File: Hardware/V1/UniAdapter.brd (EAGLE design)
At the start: 30 x 21 mm, 24 parts, among them IC1 LD1117S33TR, IC2 SN65HVD232D, IC3 STM32F072CBT6, X1 CAN Bus, X2 CAN Bus

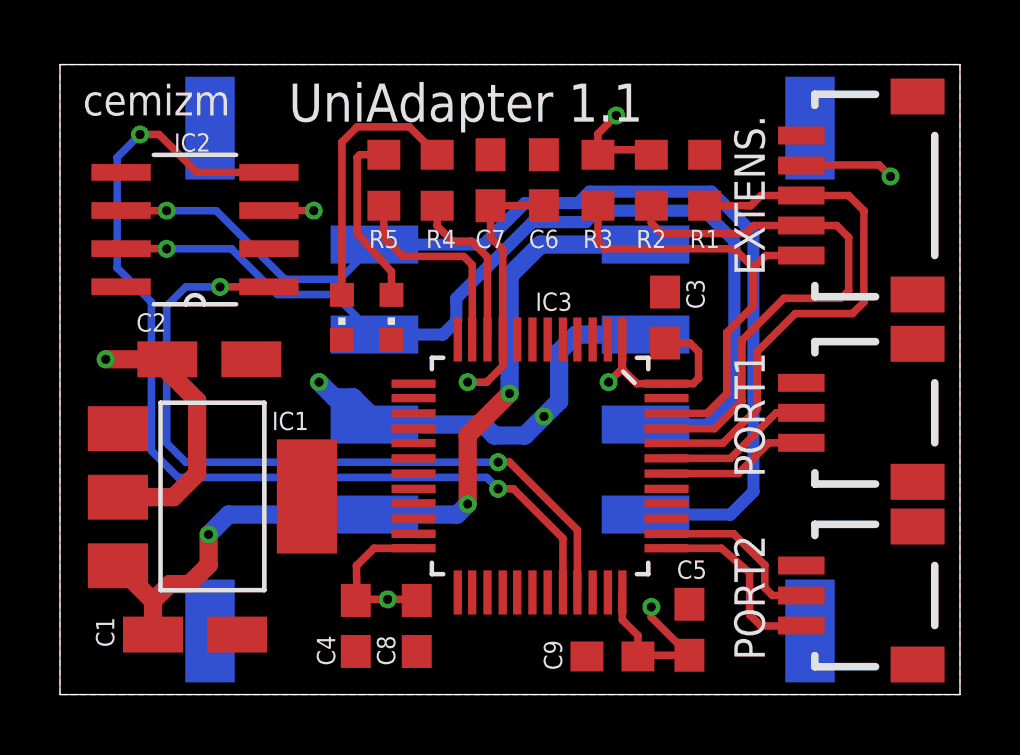
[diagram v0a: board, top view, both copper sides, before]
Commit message: AnySense 1.1
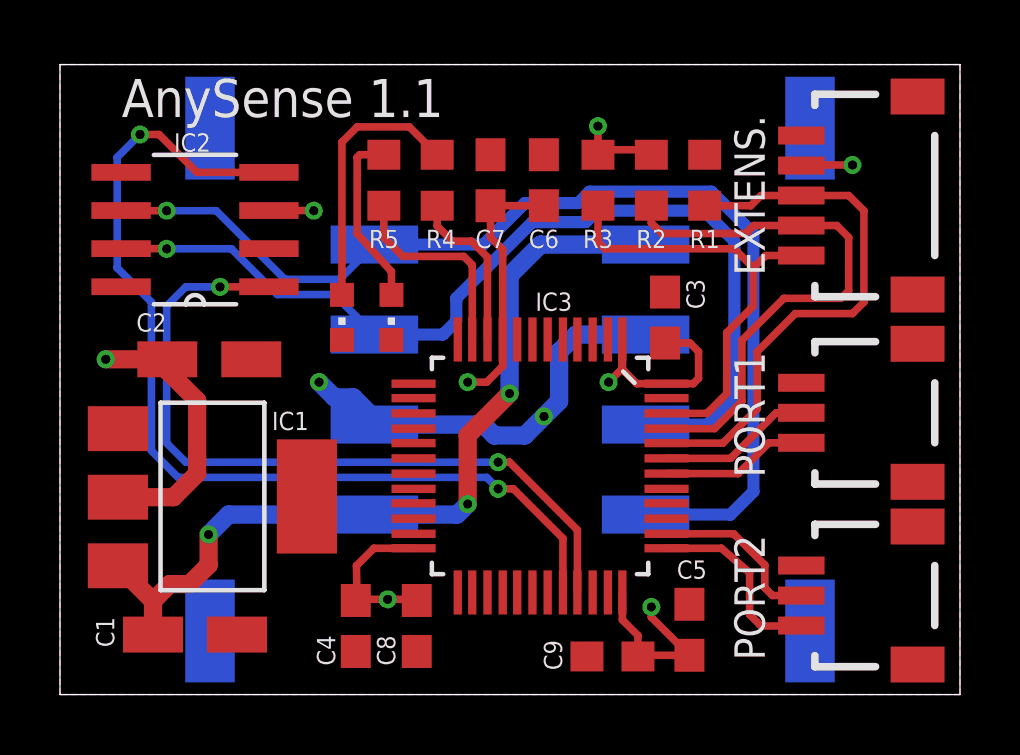
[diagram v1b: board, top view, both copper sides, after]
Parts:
- R4: value 55Ohm -> 68Ohm
- R5: value 55Ohm -> 56Ohm
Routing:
- net VCC: track 45.5 -> 43.4 mm
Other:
- board text added: "AnySense 1.1"
- board text removed: "UniAdapter 1.1"
- board text removed: "cemizm"
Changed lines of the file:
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@@
 <wire x1="22.7097375" y1="1.53345" x2="37.66655" y2="1.53345" width="0.254" layer="49"/>
 <wire x1="37.66655" y1="1.53345" x2="37.7" y2="1.5" width="0.254" layer="49" curve="-90"/>
-<text x="7.62" y="19.098" size="1.27" layer="25" font="vector">UniAdapter 1.1</text>
-<text x="0.762" y="19.304" size="1.016" layer="25" font="vector">cemizm</text>
+<text x="2.0574" y="19.2504" size="1.27" layer="25" font="vector">AnySense 1.1</text>
 </plain>
 <attributes>
@@
 <attribute name="OC_FARNELL" value="2331730" x="19.7104" y="17.145" size="1.778" layer="27" rot="R270" display="off"/>
 </element>
-<element name="R4" library="rcl" package="R0603" value="55Ohm" x="12.573" y="17.145" smashed="yes" rot="R90">
+<element name="R4" library="rcl" package="R0603" value="68Ohm" x="12.573" y="17.145" smashed="yes" rot="R90">
 <attribute name="NAME" x="12.7" y="15.494" size="0.6096" layer="25" rot="R180" align="bottom-center"/>
 <attribute name="VALUE" x="14.478" y="16.51" size="1.27" layer="27" rot="R90"/>
-</element>
-<element name="R5" library="rcl" package="R0603" value="55Ohm" x="10.795" y="17.145" smashed="yes" rot="R90">
+<attribute name="OC_FARNELL" value="2331710" x="12.573" y="17.145" size="1.778" layer="27" rot="R90" display="off"/>
+</element>
+<element name="R5" library="rcl" package="R0603" value="56Ohm" x="10.795" y="17.145" smashed="yes" rot="R90">
 <attribute name="NAME" x="10.795" y="15.494" size="0.6096" layer="25" rot="R180" align="bottom-center"/>
 <attribute name="VALUE" x="12.7" y="16.51" size="1.27" layer="27" rot="R90"/>
+<attribute name="OC_FARNELL" value="2331709" x="10.795" y="17.145" size="1.778" layer="27" rot="R90" display="off"/>
 </element>
 <element name="LD1" library="led" package="CHIPLED_0603" value="RED" x="9.398" y="12.573" smashed="yes" rot="R180">
 <attribute name="VALUE" x="7.493" y="13.843" size="1.27" layer="27" rot="R270"/>
+<attribute name="OC_FARNELL" value="2099221" x="9.398" y="12.573" size="1.778" layer="27" rot="R180" display="off"/>
 </element>
 <element name="LD2" library="led" package="CHIPLED_0603" value="GREEN" x="11.049" y="12.573" smashed="yes" rot="R180">
 <attribute name="VALUE" x="9.144" y="13.843" size="1.27" layer="27" rot="R270"/>
+<attribute name="OC_FARNELL" value="2099223" x="11.049" y="12.573" size="1.778" layer="27" rot="R180" display="off"/>
 </element>
 </elements>
@@
 <wire x1="9.906" y1="3.055" x2="9.86" y2="3.136" width="0.254" layer="1"/>
 <wire x1="24.711" y1="17.635" x2="24.729" y2="17.653" width="0.254" layer="1"/>
-<wire x1="24.729" y1="17.653" x2="27.305" y2="17.653" width="0.254" layer="1"/>
-<wire x1="27.305" y1="17.653" x2="27.686" y2="17.272" width="0.254" layer="1"/>
-<via x="27.686" y="17.272" extent="1-16" drill="0.3048"/>
+<wire x1="24.729" y1="17.653" x2="26.416" y2="17.653" width="0.254" layer="1"/>
+<via x="26.416" y="17.653" extent="1-16" drill="0.3048"/>
 <wire x1="18.7452" y1="11.8364" x2="18.7452" y2="10.8712" width="0.254" layer="1"/>
 <wire x1="18.7452" y1="10.8712" x2="18.288" y2="10.414" width="0.254" layer="1"/>
@@
 <wire x1="14.351" y1="15.24" x2="14.7574" y2="14.8336" width="0.254" layer="1"/>
 <wire x1="14.7574" y1="14.8336" x2="14.7574" y2="11.8364" width="0.254" layer="1"/>
-<wire x1="17.9324" y1="17.995" x2="17.9324" y2="18.6944" width="0.254" layer="1"/>
-<wire x1="17.9324" y1="18.6944" x2="18.542" y2="19.304" width="0.254" layer="1"/>
-<via x="18.542" y="19.304" extent="1-16" drill="0.3048"/>
+<wire x1="17.9324" y1="17.995" x2="17.9324" y2="18.9484" width="0.254" layer="1"/>
+<via x="17.9324" y="18.9484" extent="1-16" drill="0.3048"/>
 </signal>
 <signal name="CANRX">

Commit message: Revert "AnySense 1.1"
This reverts commit 53d5508880b3b2ed964bc1ff9d3bc3f9eadd301f.
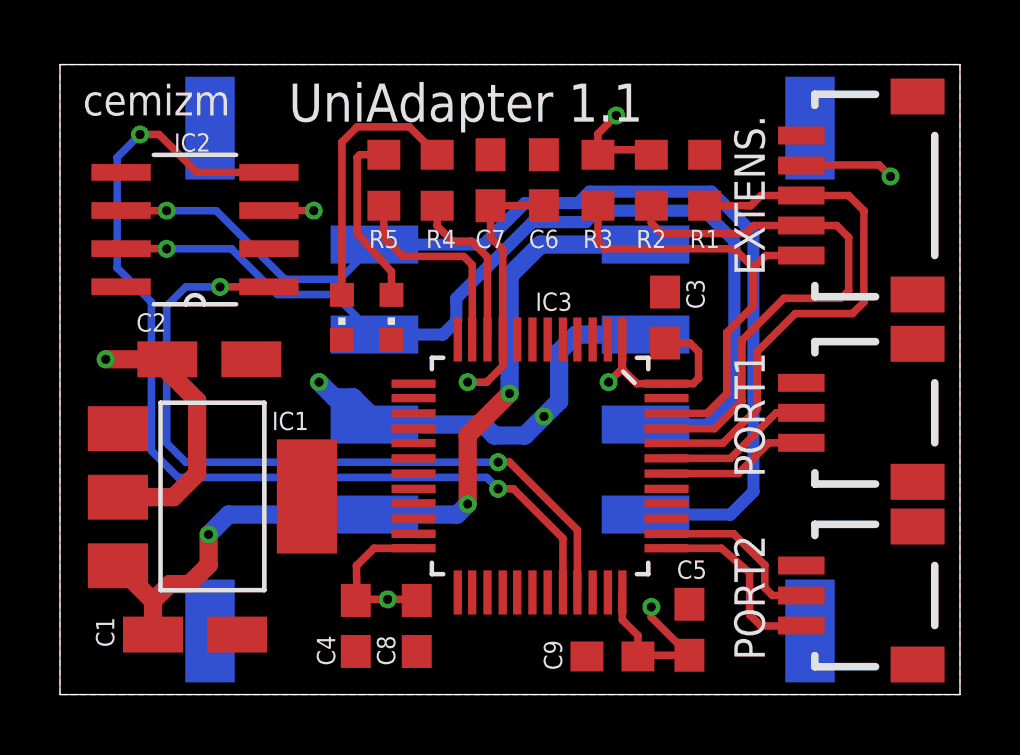
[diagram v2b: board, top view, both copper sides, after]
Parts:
- R4: value 68Ohm -> 55Ohm
- R5: value 56Ohm -> 55Ohm
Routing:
- net VCC: track 43.4 -> 45.5 mm
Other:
- board text added: "UniAdapter 1.1"
- board text added: "cemizm"
- board text removed: "AnySense 1.1"
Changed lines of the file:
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@@
 <wire x1="22.7097375" y1="1.53345" x2="37.66655" y2="1.53345" width="0.254" layer="49"/>
 <wire x1="37.66655" y1="1.53345" x2="37.7" y2="1.5" width="0.254" layer="49" curve="-90"/>
-<text x="2.0574" y="19.2504" size="1.27" layer="25" font="vector">AnySense 1.1</text>
+<text x="7.62" y="19.098" size="1.27" layer="25" font="vector">UniAdapter 1.1</text>
+<text x="0.762" y="19.304" size="1.016" layer="25" font="vector">cemizm</text>
 </plain>
 <attributes>
@@
 <attribute name="OC_FARNELL" value="2331730" x="19.7104" y="17.145" size="1.778" layer="27" rot="R270" display="off"/>
 </element>
-<element name="R4" library="rcl" package="R0603" value="68Ohm" x="12.573" y="17.145" smashed="yes" rot="R90">
+<element name="R4" library="rcl" package="R0603" value="55Ohm" x="12.573" y="17.145" smashed="yes" rot="R90">
 <attribute name="NAME" x="12.7" y="15.494" size="0.6096" layer="25" rot="R180" align="bottom-center"/>
 <attribute name="VALUE" x="14.478" y="16.51" size="1.27" layer="27" rot="R90"/>
-<attribute name="OC_FARNELL" value="2331710" x="12.573" y="17.145" size="1.778" layer="27" rot="R90" display="off"/>
-</element>
-<element name="R5" library="rcl" package="R0603" value="56Ohm" x="10.795" y="17.145" smashed="yes" rot="R90">
+</element>
+<element name="R5" library="rcl" package="R0603" value="55Ohm" x="10.795" y="17.145" smashed="yes" rot="R90">
 <attribute name="NAME" x="10.795" y="15.494" size="0.6096" layer="25" rot="R180" align="bottom-center"/>
 <attribute name="VALUE" x="12.7" y="16.51" size="1.27" layer="27" rot="R90"/>
-<attribute name="OC_FARNELL" value="2331709" x="10.795" y="17.145" size="1.778" layer="27" rot="R90" display="off"/>
 </element>
 <element name="LD1" library="led" package="CHIPLED_0603" value="RED" x="9.398" y="12.573" smashed="yes" rot="R180">
 <attribute name="VALUE" x="7.493" y="13.843" size="1.27" layer="27" rot="R270"/>
-<attribute name="OC_FARNELL" value="2099221" x="9.398" y="12.573" size="1.778" layer="27" rot="R180" display="off"/>
 </element>
 <element name="LD2" library="led" package="CHIPLED_0603" value="GREEN" x="11.049" y="12.573" smashed="yes" rot="R180">
 <attribute name="VALUE" x="9.144" y="13.843" size="1.27" layer="27" rot="R270"/>
-<attribute name="OC_FARNELL" value="2099223" x="11.049" y="12.573" size="1.778" layer="27" rot="R180" display="off"/>
 </element>
 </elements>
@@
 <wire x1="9.906" y1="3.055" x2="9.86" y2="3.136" width="0.254" layer="1"/>
 <wire x1="24.711" y1="17.635" x2="24.729" y2="17.653" width="0.254" layer="1"/>
-<wire x1="24.729" y1="17.653" x2="26.416" y2="17.653" width="0.254" layer="1"/>
-<via x="26.416" y="17.653" extent="1-16" drill="0.3048"/>
+<wire x1="24.729" y1="17.653" x2="27.305" y2="17.653" width="0.254" layer="1"/>
+<wire x1="27.305" y1="17.653" x2="27.686" y2="17.272" width="0.254" layer="1"/>
+<via x="27.686" y="17.272" extent="1-16" drill="0.3048"/>
 <wire x1="18.7452" y1="11.8364" x2="18.7452" y2="10.8712" width="0.254" layer="1"/>
 <wire x1="18.7452" y1="10.8712" x2="18.288" y2="10.414" width="0.254" layer="1"/>
@@
 <wire x1="14.351" y1="15.24" x2="14.7574" y2="14.8336" width="0.254" layer="1"/>
 <wire x1="14.7574" y1="14.8336" x2="14.7574" y2="11.8364" width="0.254" layer="1"/>
-<wire x1="17.9324" y1="17.995" x2="17.9324" y2="18.9484" width="0.254" layer="1"/>
-<via x="17.9324" y="18.9484" extent="1-16" drill="0.3048"/>
+<wire x1="17.9324" y1="17.995" x2="17.9324" y2="18.6944" width="0.254" layer="1"/>
+<wire x1="17.9324" y1="18.6944" x2="18.542" y2="19.304" width="0.254" layer="1"/>
+<via x="18.542" y="19.304" extent="1-16" drill="0.3048"/>
 </signal>
 <signal name="CANRX">
